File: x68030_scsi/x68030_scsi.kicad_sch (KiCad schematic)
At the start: 43 parts, among them J1 Conn_02x25_Odd_Even, J2 Conn_02x20_Odd_Even, J3 Conn_02x03_Odd_Even

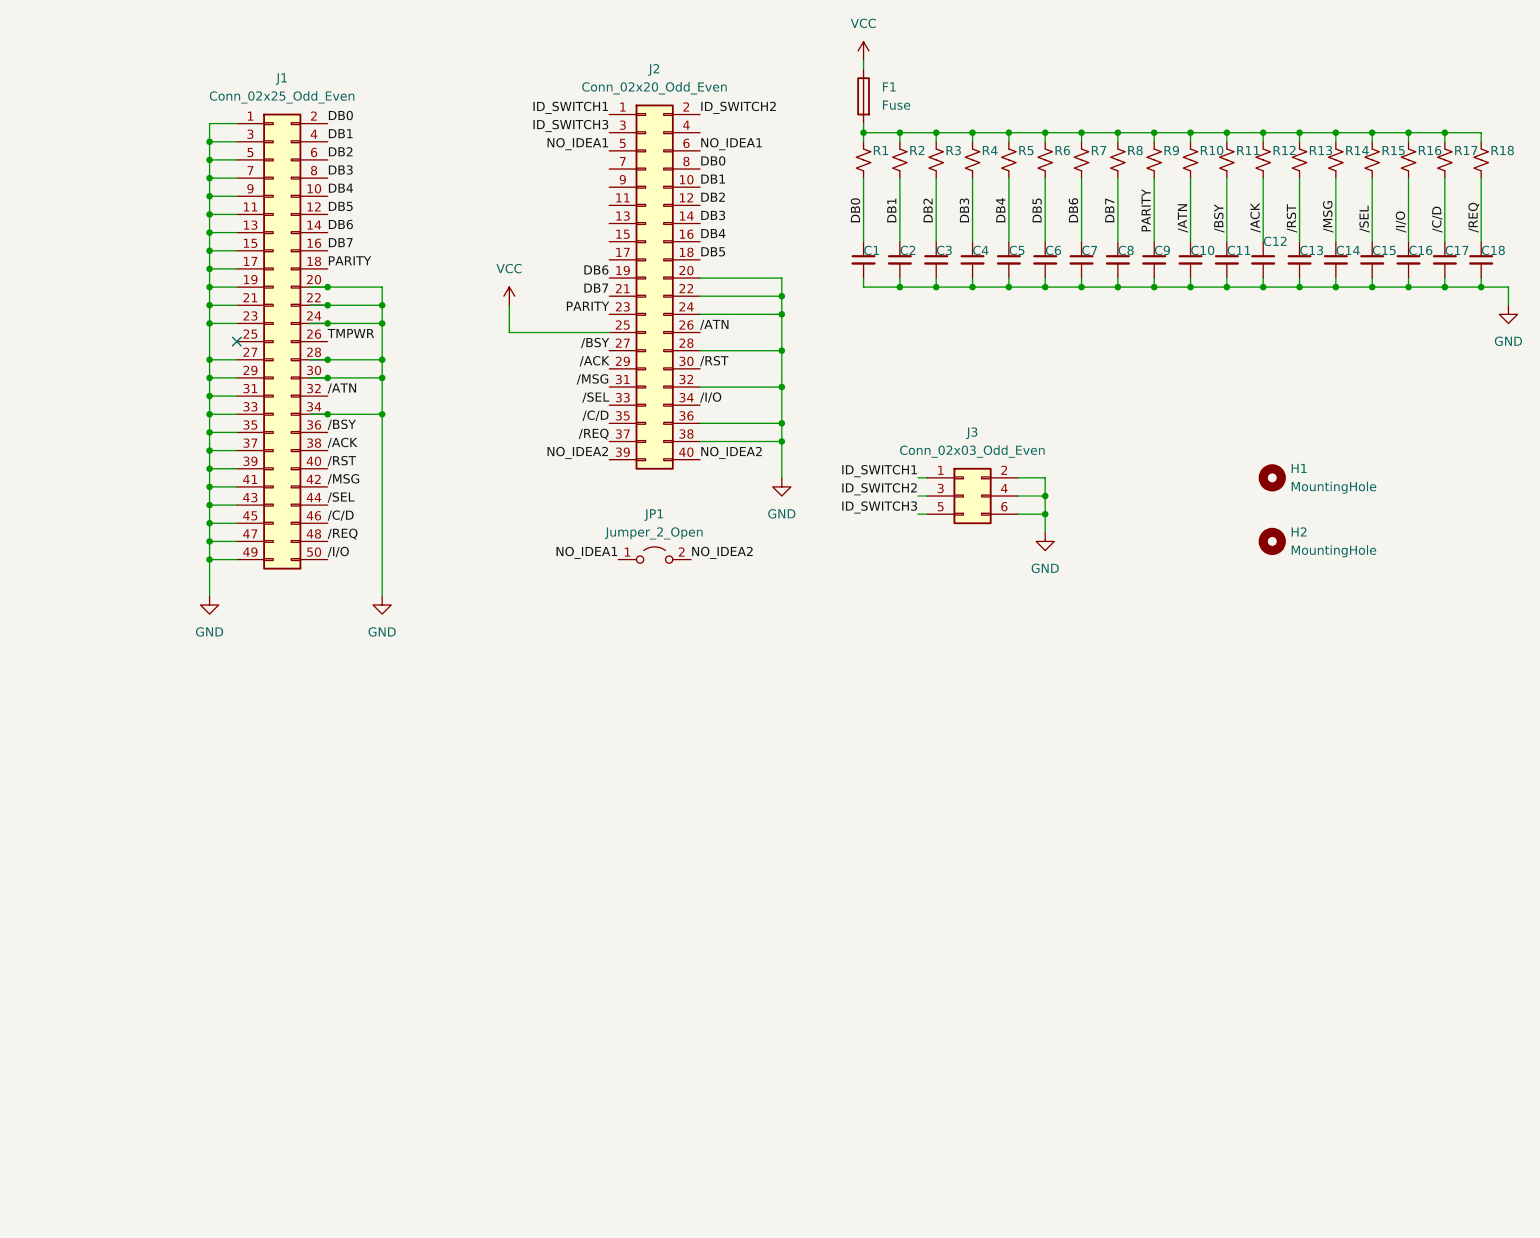
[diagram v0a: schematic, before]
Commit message: fixes
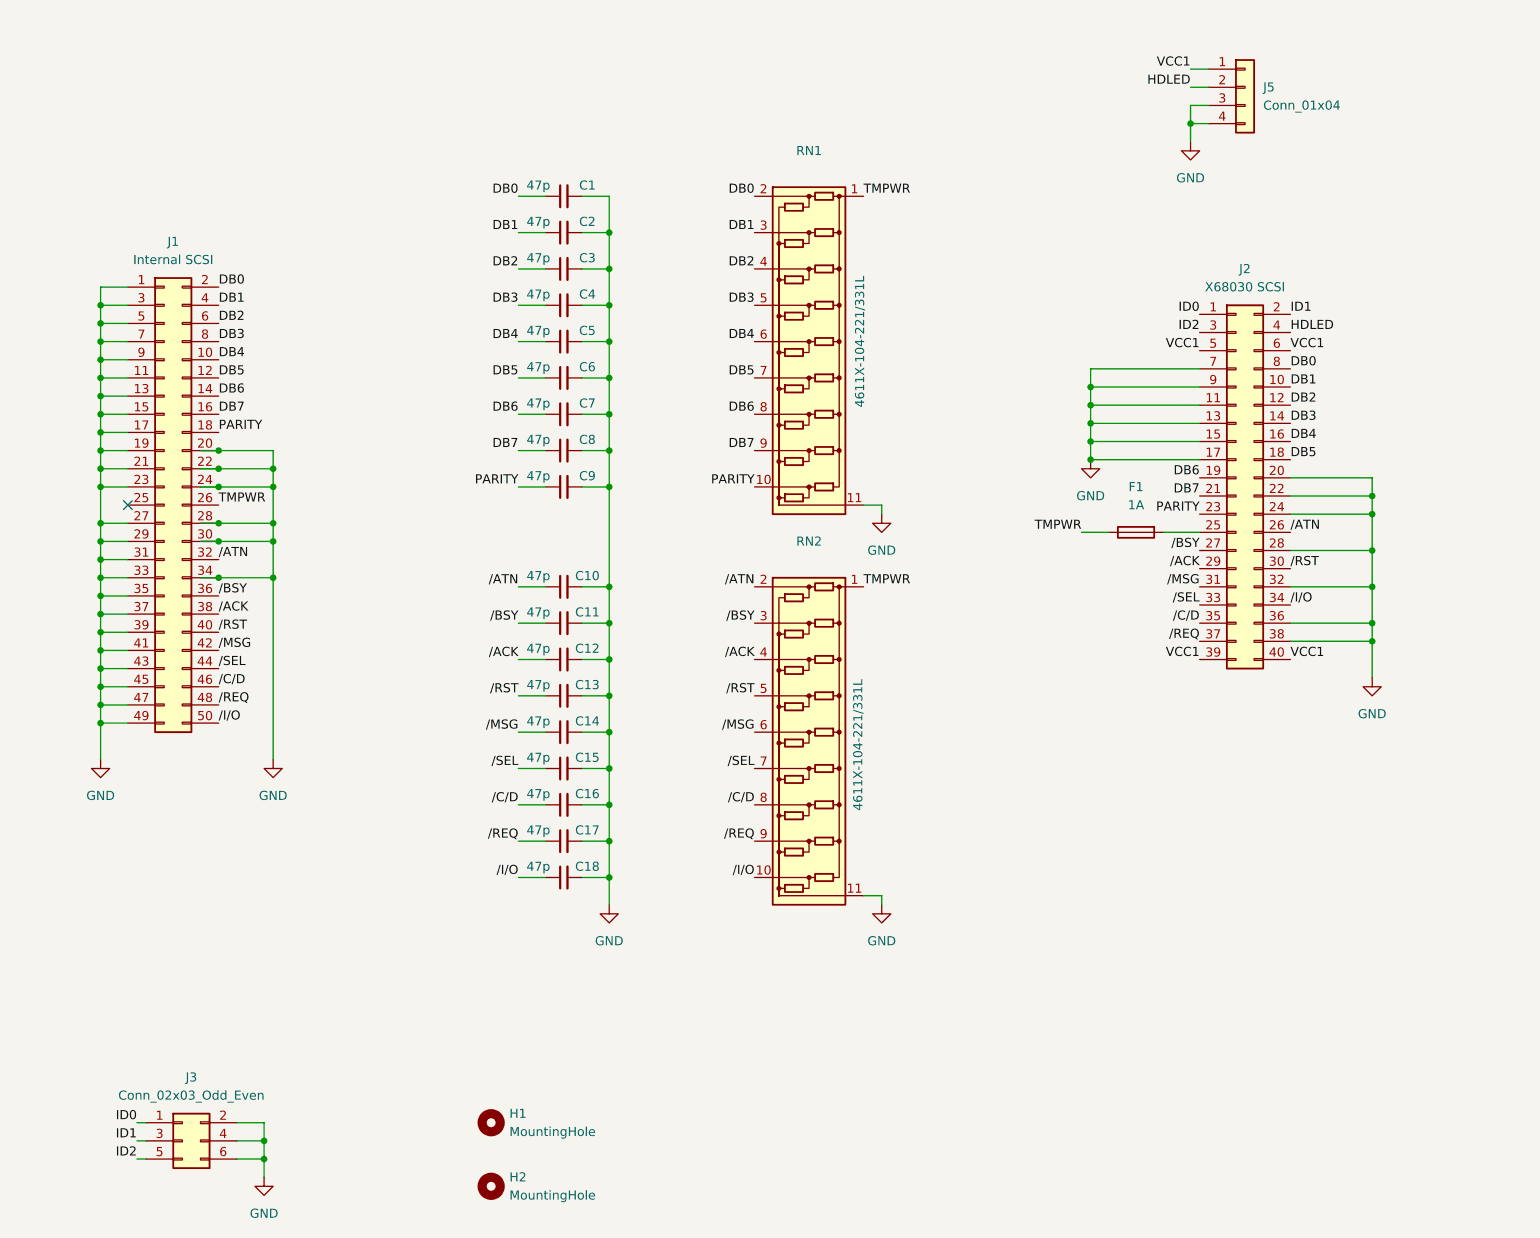
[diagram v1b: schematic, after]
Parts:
- removed JP1: Jumper_2_Open, Resistor_SMD:R_0603_1608Metric_Pad0.98x0.95mm_HandSolder, symbol Jumper:Jumper_2_Open
- removed R1, R10, R11, R12, R13, R14, R15, R16, R17, R18, R2, R3, R4, R5, R6, R7, R8, R9: R_Small_US, Resistor_SMD:R_0603_1608Metric_Pad0.98x0.95mm_HandSolder, symbol Device:R_Small_US
- added J5: Conn_01x04, Connector_PinHeader_2.54mm:PinHeader_1x04_P2.54mm_Horizontal, symbol Connector_Generic:Conn_01x04
- added RN1, RN2: 4611X-104-221/331L, Resistor_THT:R_Array_SIP11, symbol Device:R_Network_Dividers_x09_SIP
- C1, C10, C11, C12, C13, C14, C15, C16, C17, C18, C2, C3, C4, C5, C6, C7, C8, C9: value C_Small -> 47p; footprint Capacitor_SMD:C_0603_1608Metric_Pad1.08x0.95mm_HandSolder -> Capacitor_SMD:C_0805_2012Metric_Pad1.18x1.45mm_HandSolder; Mouser (none) -> 80-C0805X470J1HACTU
- F1: value Fuse -> 1A; footprint Fuse:Fuse_0603_1608Metric_Pad1.05x0.95mm_HandSolder -> Fuse:Fuse_0805_2012Metric_Pad1.15x1.40mm_HandSolder; Mouser (none) -> 594-MFU0805-FF-1.0
- J1: value Conn_02x25_Odd_Even -> Internal SCSI
- J2: value Conn_02x20_Odd_Even -> X68030 SCSI
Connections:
- net NO_IDEA2 is gone; now on net VCC1: J2.39 (Pin_39), J2.40 (Pin_40)
- net DB0: now also RN1.2 (R1)
- net DB1: now also RN1.3 (R2)
- net DB2: now also RN1.4 (R3)
- net DB3: now also RN1.5 (R4)
- net DB4: now also RN1.6 (R5)
- net DB5: now also RN1.7 (R6)
- net DB6: now also RN1.8 (R7)
- net DB7: now also RN1.9 (R8)
- net GND: now also J2.11 (Pin_11), J2.13 (Pin_13), J2.15 (Pin_15), J2.17 (Pin_17), J2.7 (Pin_7), J2.9 (Pin_9), J5.3 (Pin_3), J5.4 (Pin_4), RN1.11 (COM2), RN2.11 (COM2)
- net PARITY: now also RN1.10 (R9)
- net TMPWR: now also F1.1, RN1.1 (COM1), RN2.1 (COM1)
- net /ACK: now also RN2.4 (R3)
- net /ATN: now also RN2.2 (R1)
- net /BSY: now also RN2.3 (R2)
- net /C/D: now also C16.1, RN2.8 (R7); no longer C17.1
- net /I/O: now also C18.1, RN2.10 (R9); no longer C16.1
- net /MSG: now also RN2.6 (R5)
- net /REQ: now also C17.1, RN2.9 (R8); no longer C18.1
- net /RST: now also RN2.5 (R4)
- net /SEL: now also RN2.7 (R6)
- net at F1.2: now also J2.25 (Pin_25)
- net HDLED: now reaches J2.4 (Pin_4)
- net HDLED: now also J5.2 (Pin_2)
- net ID_SWITCH1 renamed ID0
- net ID_SWITCH2 renamed ID1
- net ID_SWITCH3 renamed ID2
- net NO_IDEA1 renamed VCC1
- net VCC1: now also J5.1 (Pin_1)
- removed net VCC: F1.1, J2.25 (Pin_25)
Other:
- moved on the sheet: F1, H1, H2, J1, J2, J3

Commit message: Update x68030_scsi.kicad_sch
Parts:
- J1: Mouser (none) -> 737-BHR-50-VUA
- J2: Mouser (none) -> 538-87831-4021
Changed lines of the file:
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@@
+			)
+		)
+		(property "Mouser" "737-BHR-50-VUA "
+			(at 81.28 88.9 0)
+			(effects
+				(font
+					(size 1.27 1.27)
+				)
+				(hide yes)
 			)
 		)
@@
 			(at 231.14 85.09 0)
 			(effects
+				(font
+					(size 1.27 1.27)
+				)
+				(hide yes)
+			)
+		)
+		(property "Mouser" "538-87831-4021  "
+			(at 231.14 85.09 0)
+			(effects

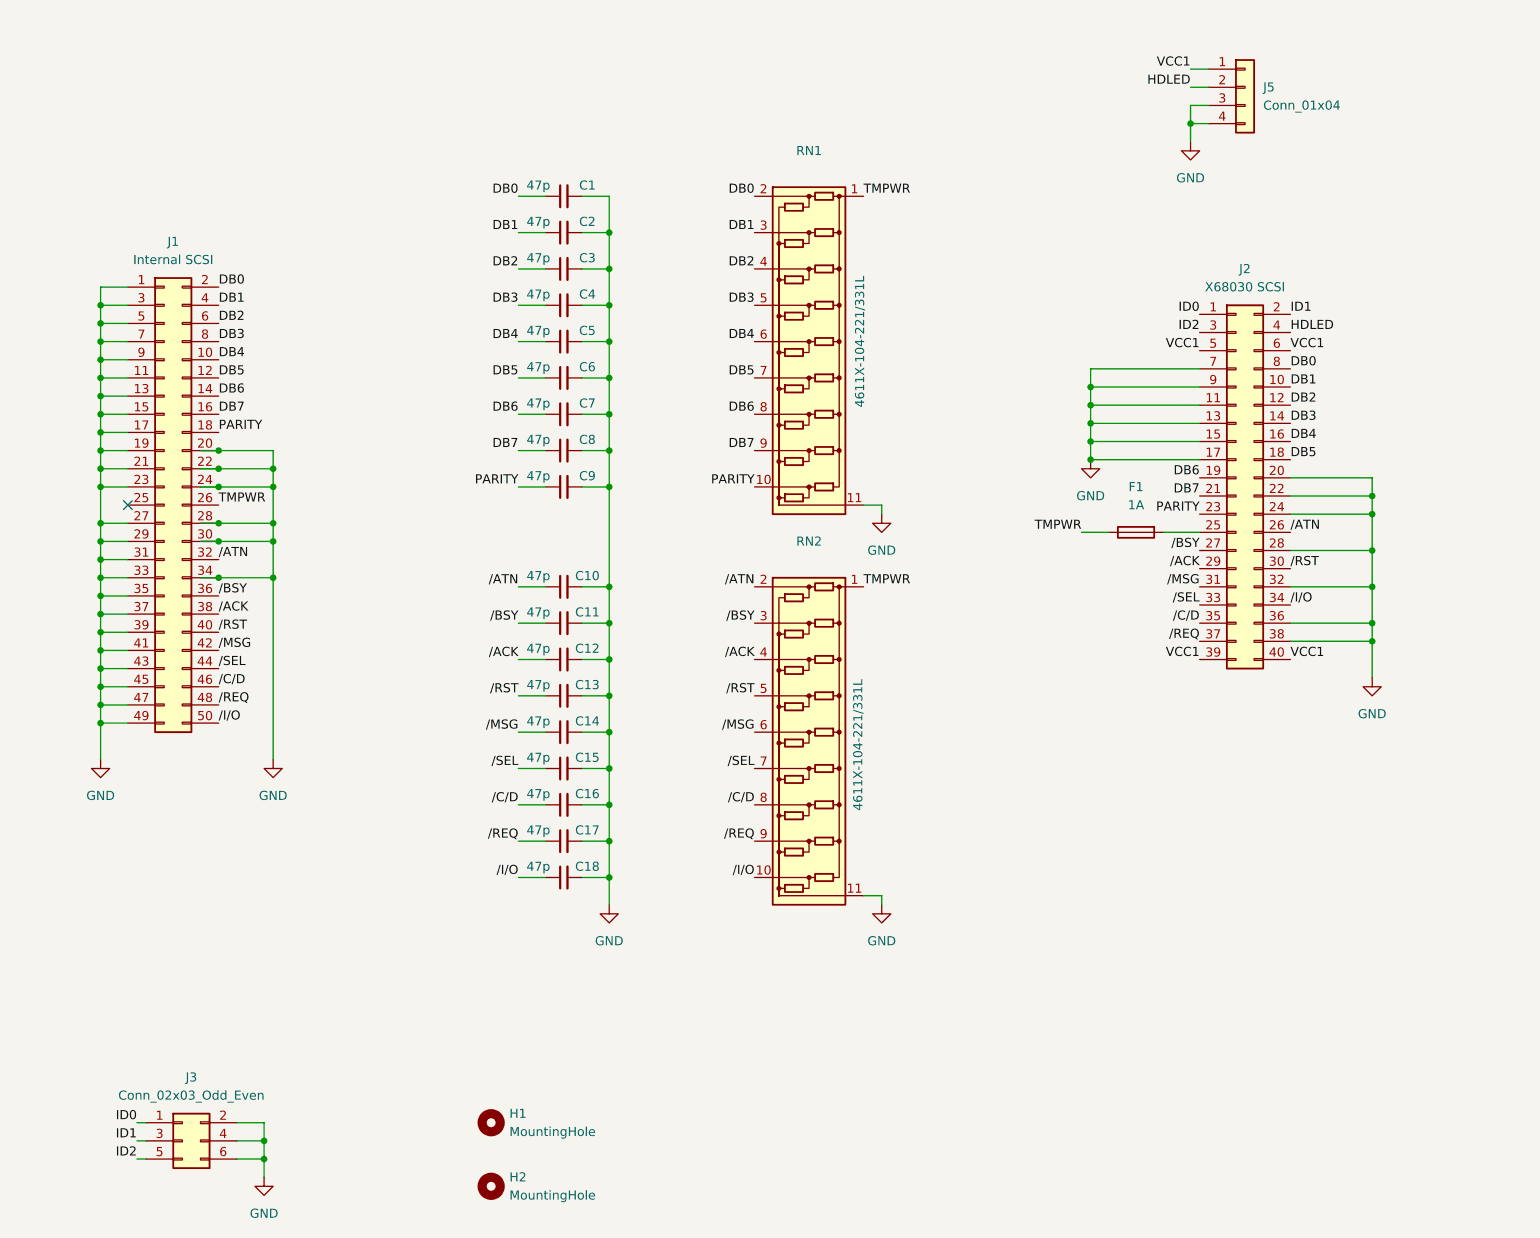
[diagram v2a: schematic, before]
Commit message: minor fixes
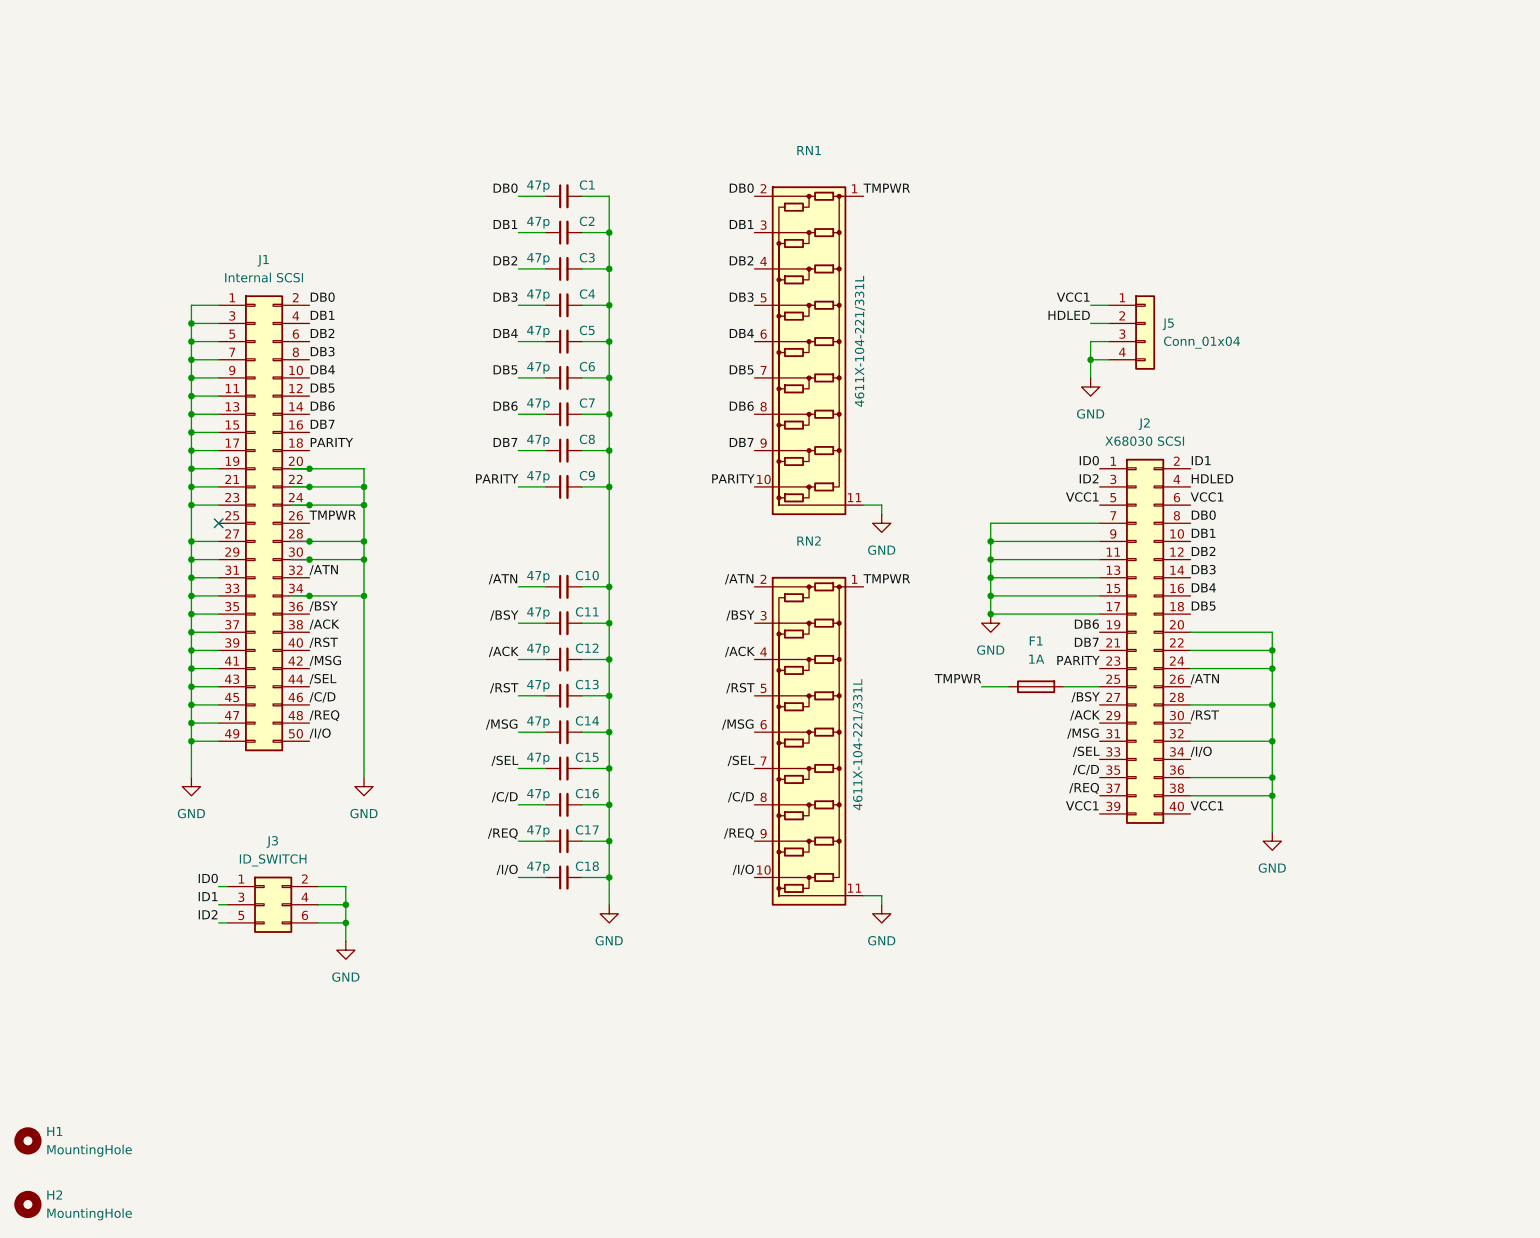
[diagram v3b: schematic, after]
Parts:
- J3: value Conn_02x03_Odd_Even -> ID_SWITCH
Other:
- moved on the sheet: F1, H1, H2, J1, J2, J3, J5
